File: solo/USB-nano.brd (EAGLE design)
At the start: 13 x 10.6 mm, 18 parts, among them U1 USB_TRACES_NANO

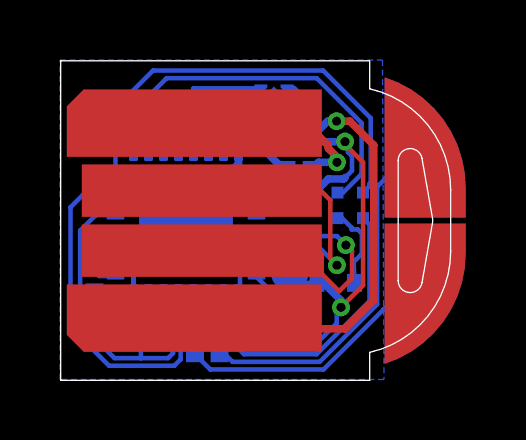
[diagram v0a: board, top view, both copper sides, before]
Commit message: Update USB-nano.brd
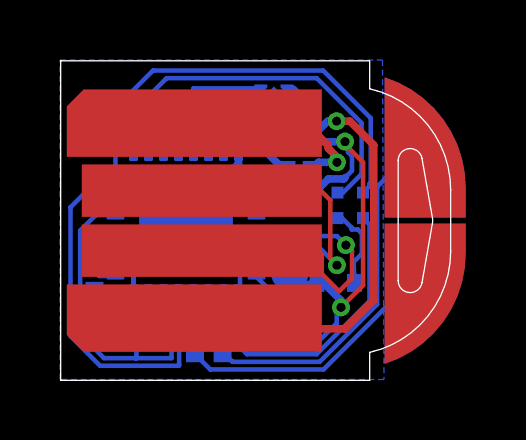
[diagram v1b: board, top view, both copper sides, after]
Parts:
- moved C3 0.80 mm to (1.27, 12.3)
- moved C1 0.20 mm to (1.89, 11.5)
- moved R2 0.10 mm to (4.82, 11.7)
- moved SWDIO 0.05 mm to (5.99, 12.3)
